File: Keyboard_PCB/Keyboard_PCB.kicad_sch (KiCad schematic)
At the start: 29 parts, among them J1 JTAG, SW1 BTN, SW2 BTN, SW3 RotaryEncoder_Switch_MP, U1 STM32F412CGUx, Y1 25MHz, Y2 32.768 KHz

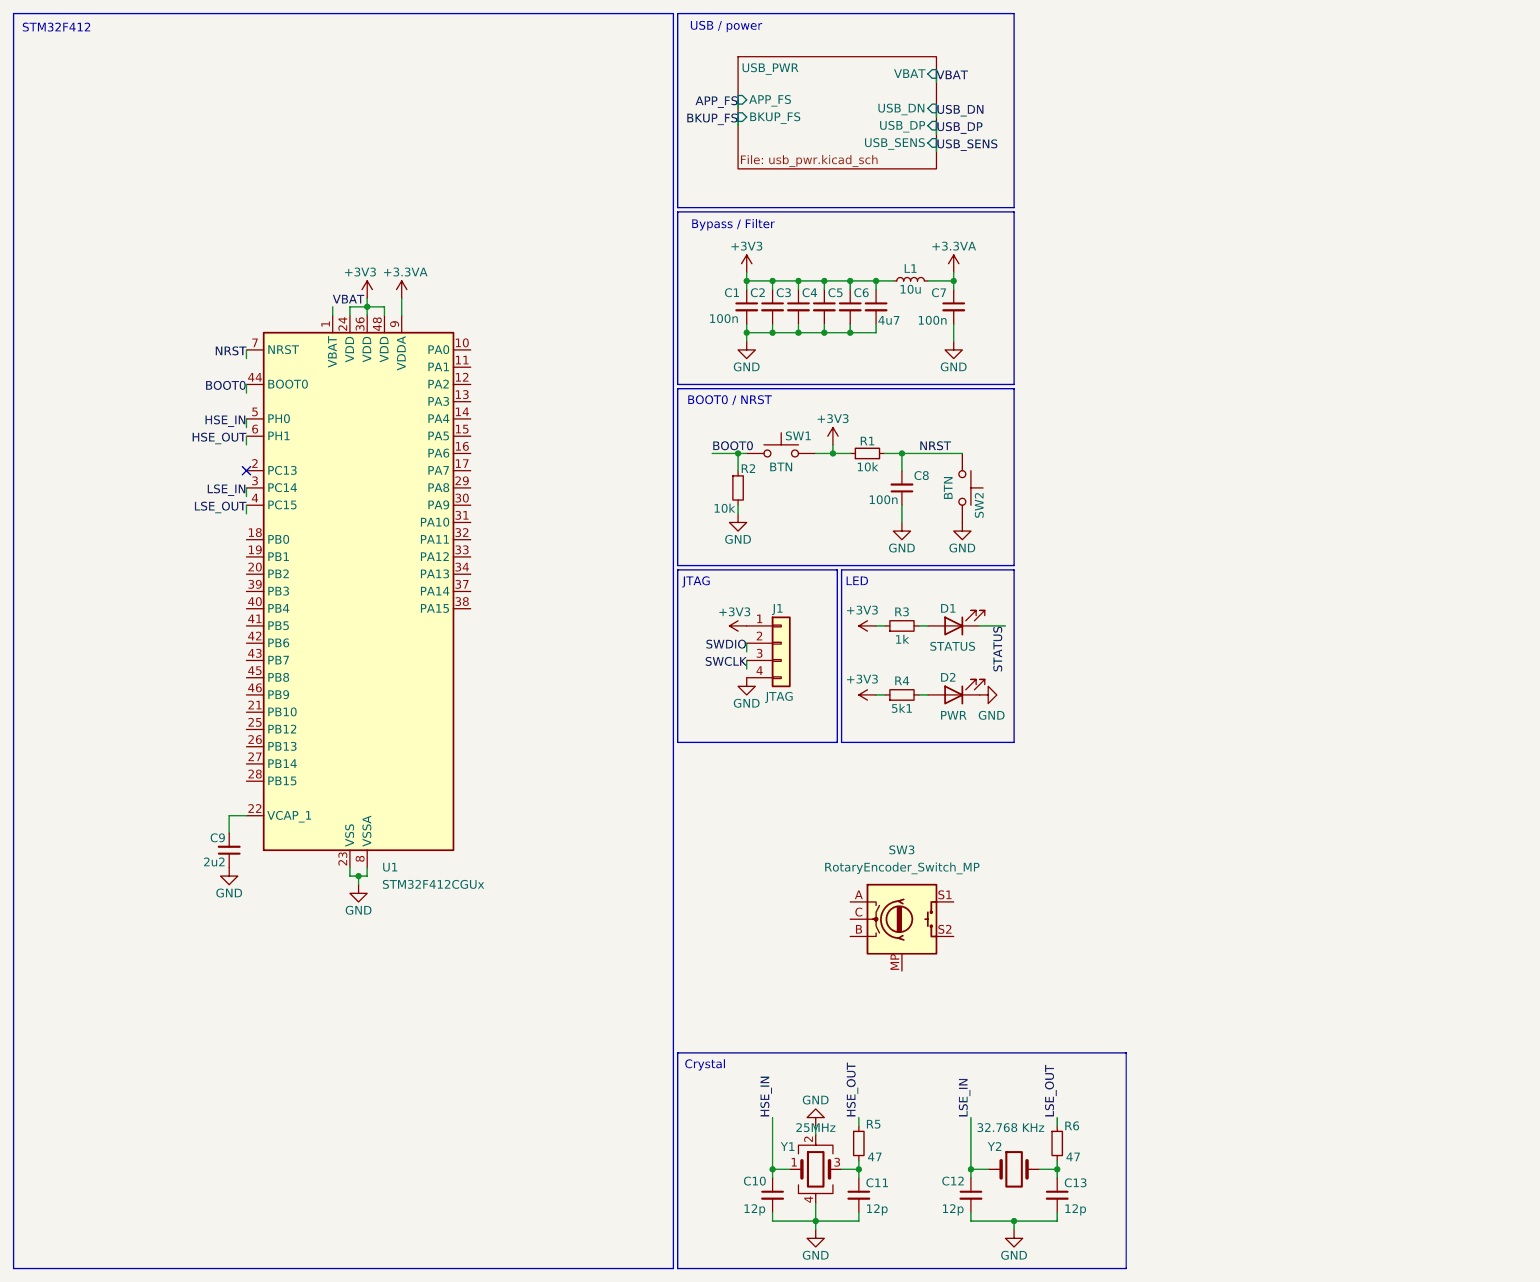
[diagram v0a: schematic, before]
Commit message: Progress
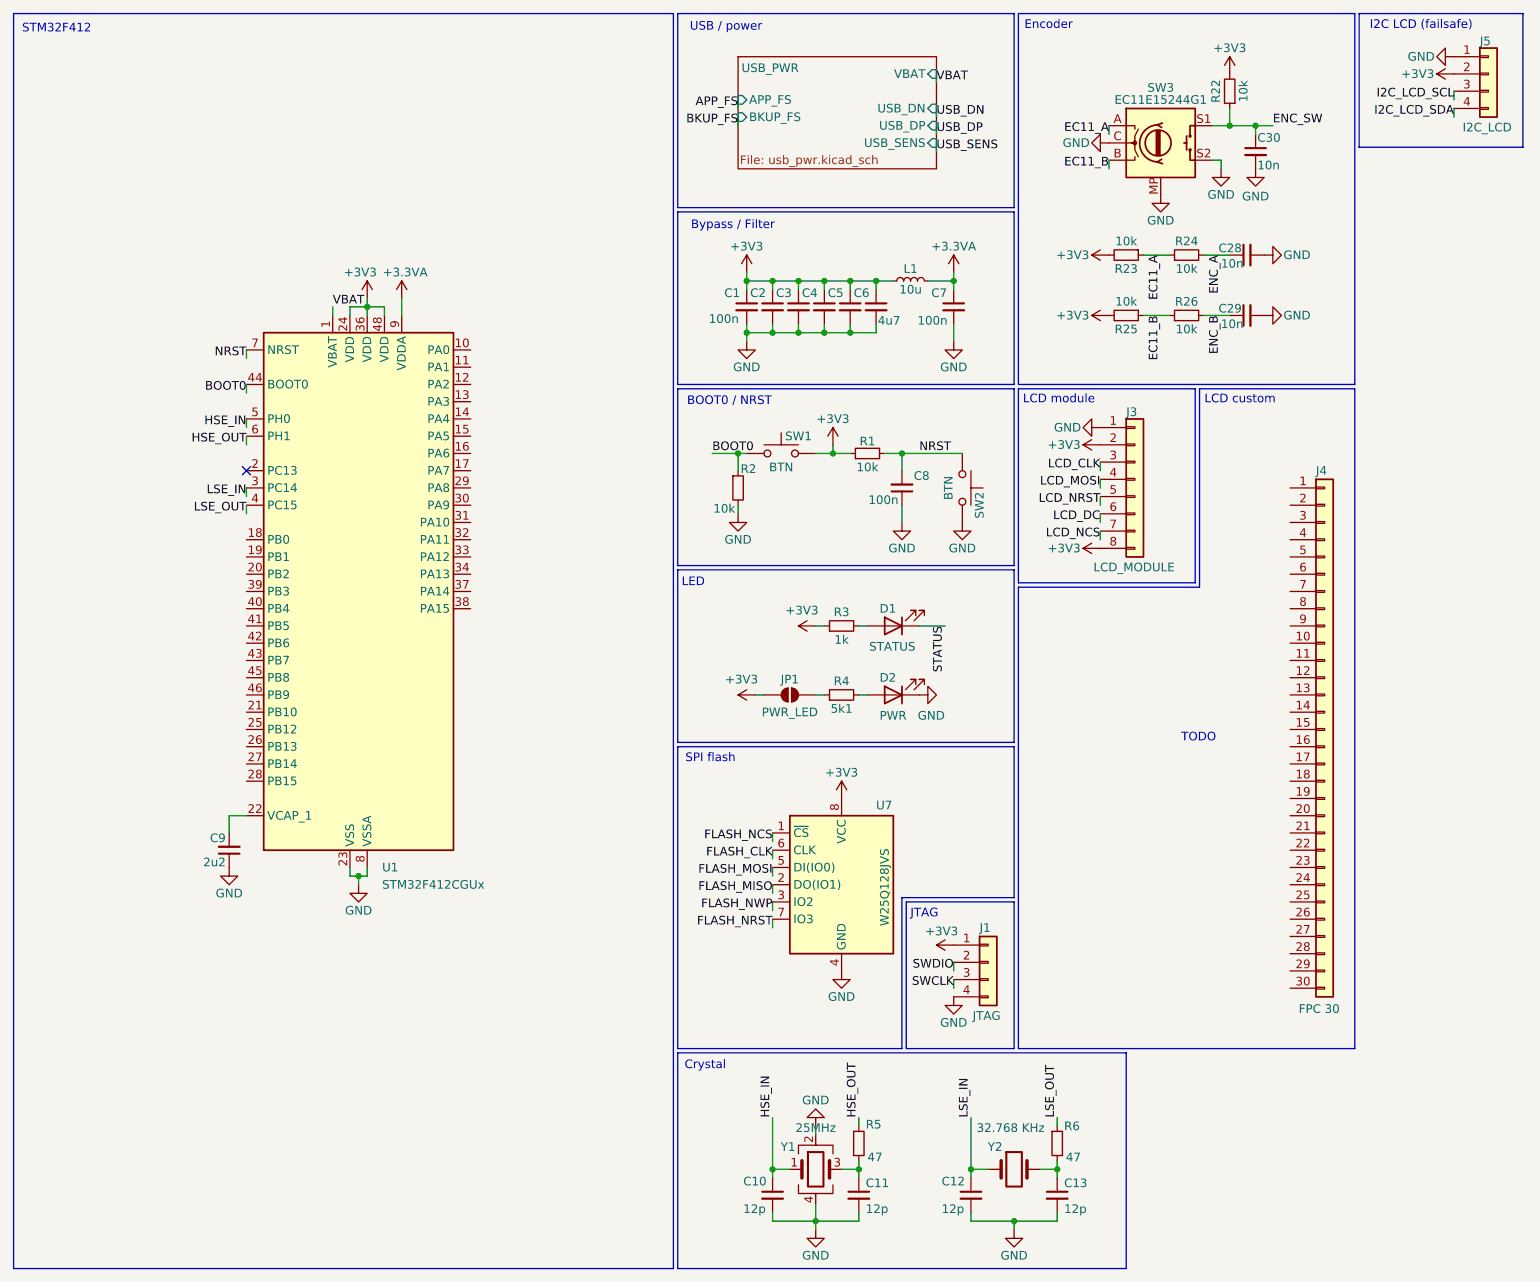
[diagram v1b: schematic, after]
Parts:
- added C28, C29, C30: 10n, Capacitor_SMD:C_0603_1608Metric, symbol Device:C_Small
- added J3: LCD_MODULE, symbol Connector_Generic:Conn_01x08
- added J4: FPC 30, symbol Connector_Generic:Conn_01x30
- added J5: I2C_LCD, symbol Connector_Generic:Conn_01x04
- added JP1: PWR_LED, symbol Jumper:SolderJumper_2_Open
- added R22, R23, R24, R25, R26: 10k, Resistor_SMD:R_0603_1608Metric, symbol Device:R_Small
- added U7: W25Q128JVS, Marijn_KiCad:SOIC-8_W25QxJVS, symbol Memory_Flash:W25Q128JVS
- SW3: value RotaryEncoder_Switch_MP -> EC11E15244G1
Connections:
- net +3V3: now also J3.2 (Pin_2), J3.8 (Pin_8), J5.2 (Pin_2), JP1.1 (A), R22.2, R23.2, R25.2, U7.8 (VCC); no longer R4.1
- net GND: now also SW3.C, SW3.MP, SW3.S2, C28.2, C29.2, C30.2, J3.1 (Pin_1), J5.1 (Pin_1), U7.4 (GND)
- net EC11_A: now reaches SW3.A
- net EC11_A: now also R23.1, R24.1
- net EC11_B: now reaches SW3.B
- net EC11_B: now also R25.1, R26.1
- net ENC_SW: now reaches SW3.S1
- net ENC_SW: now also C30.1, R22.1
- new net: JP1.2 (B), R4.1
- new net ENC_A: C28.1, R24.2
- new net ENC_B: C29.1, R26.2
- new net FLASH_CLK: U7.6 (CLK)
- new net FLASH_MISO: U7.2 (DO(IO1))
- new net FLASH_MOSI: U7.5 (DI(IO0))
- new net FLASH_NCS: U7.1 (~{CS})
- new net FLASH_NRST: U7.7 (IO3)
- new net FLASH_NWP: U7.3 (IO2)
- new net I2C_LCD_SCL: J5.3 (Pin_3)
- new net I2C_LCD_SDA: J5.4 (Pin_4)
- new net LCD_CLK: J3.3 (Pin_3)
- new net LCD_DC: J3.6 (Pin_6)
- new net LCD_MOSI: J3.4 (Pin_4)
- new net LCD_NCS: J3.7 (Pin_7)
- new net LCD_NRST: J3.5 (Pin_5)
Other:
- note added: "Encoder"
- note added: "I2C LCD (failsafe)"
- note added: "LCD custom"
- note added: "LCD module"
- note added: "SPI flash"
- note added: "TODO"
- moved on the sheet: D1, D2, J1, R3, R4, SW3
